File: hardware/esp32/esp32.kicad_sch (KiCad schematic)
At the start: 12 parts, among them J1 Conn_01x02, J2 Conn_01x02, J6 Conn_01x08, U2 ESP32-S3-MINI-1-N8

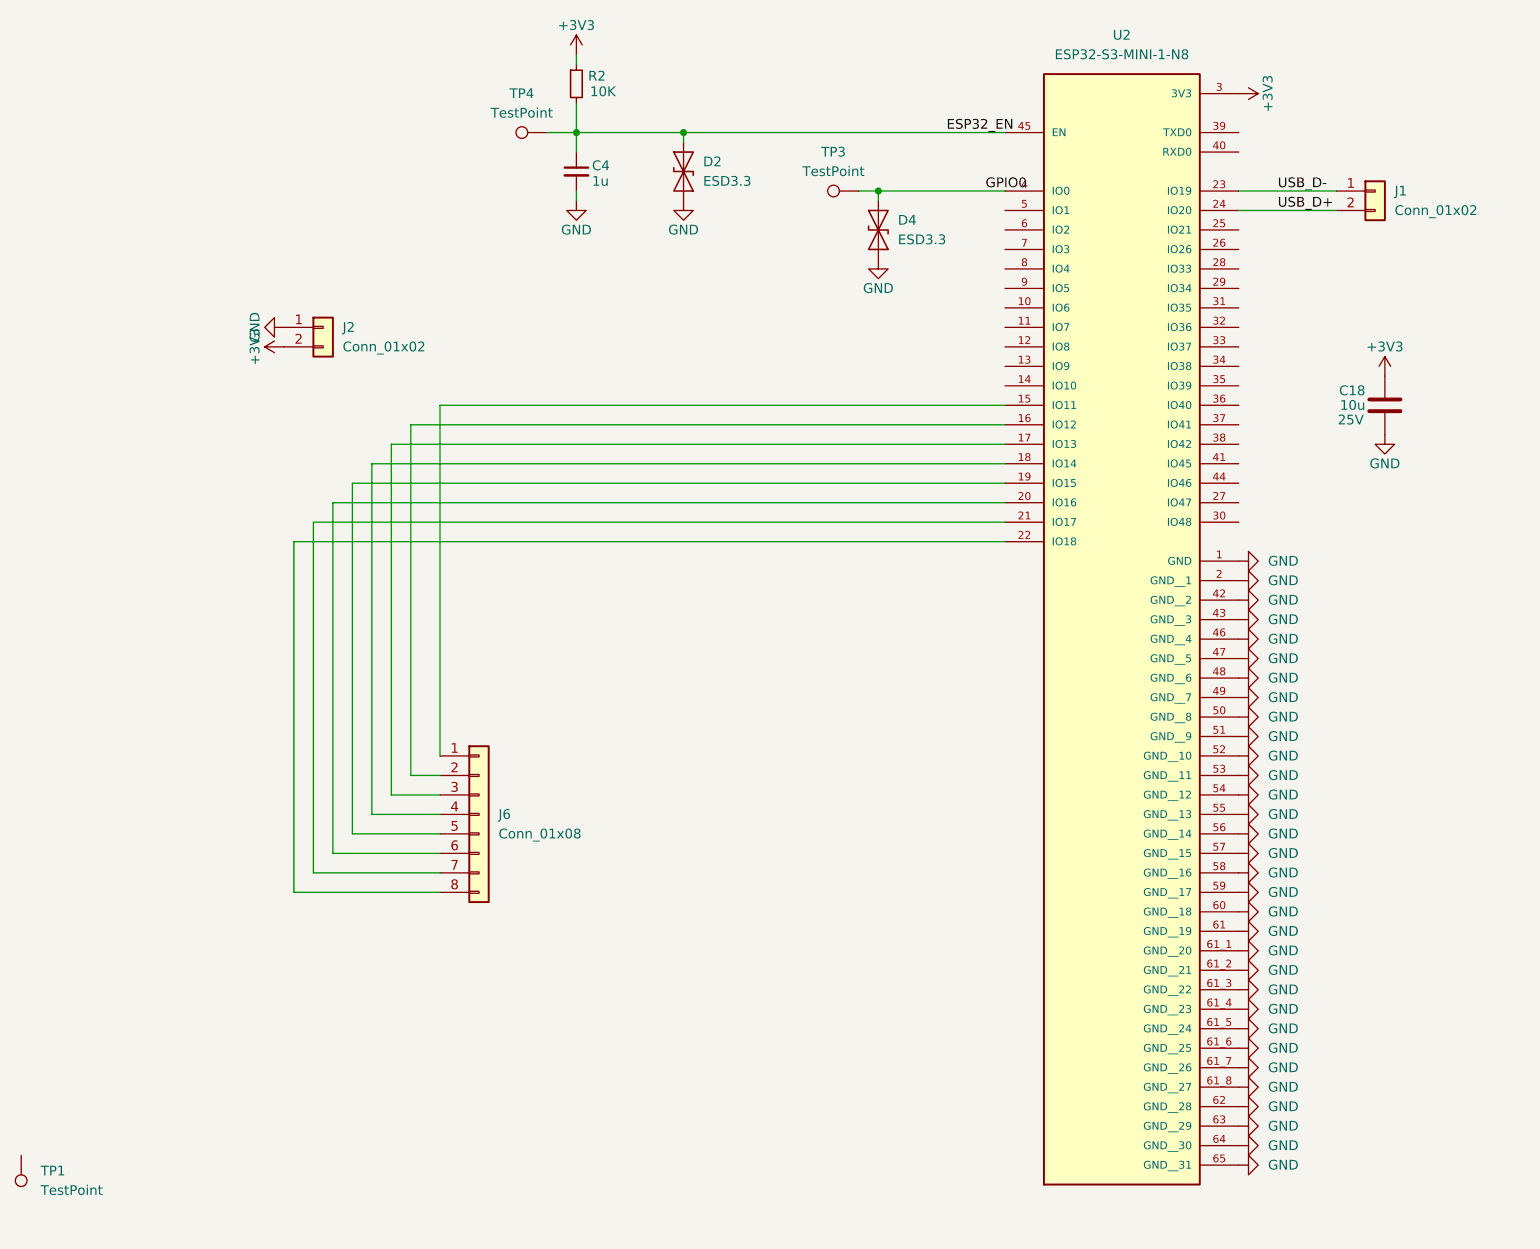
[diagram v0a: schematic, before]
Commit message: esp32 rebuild connectors
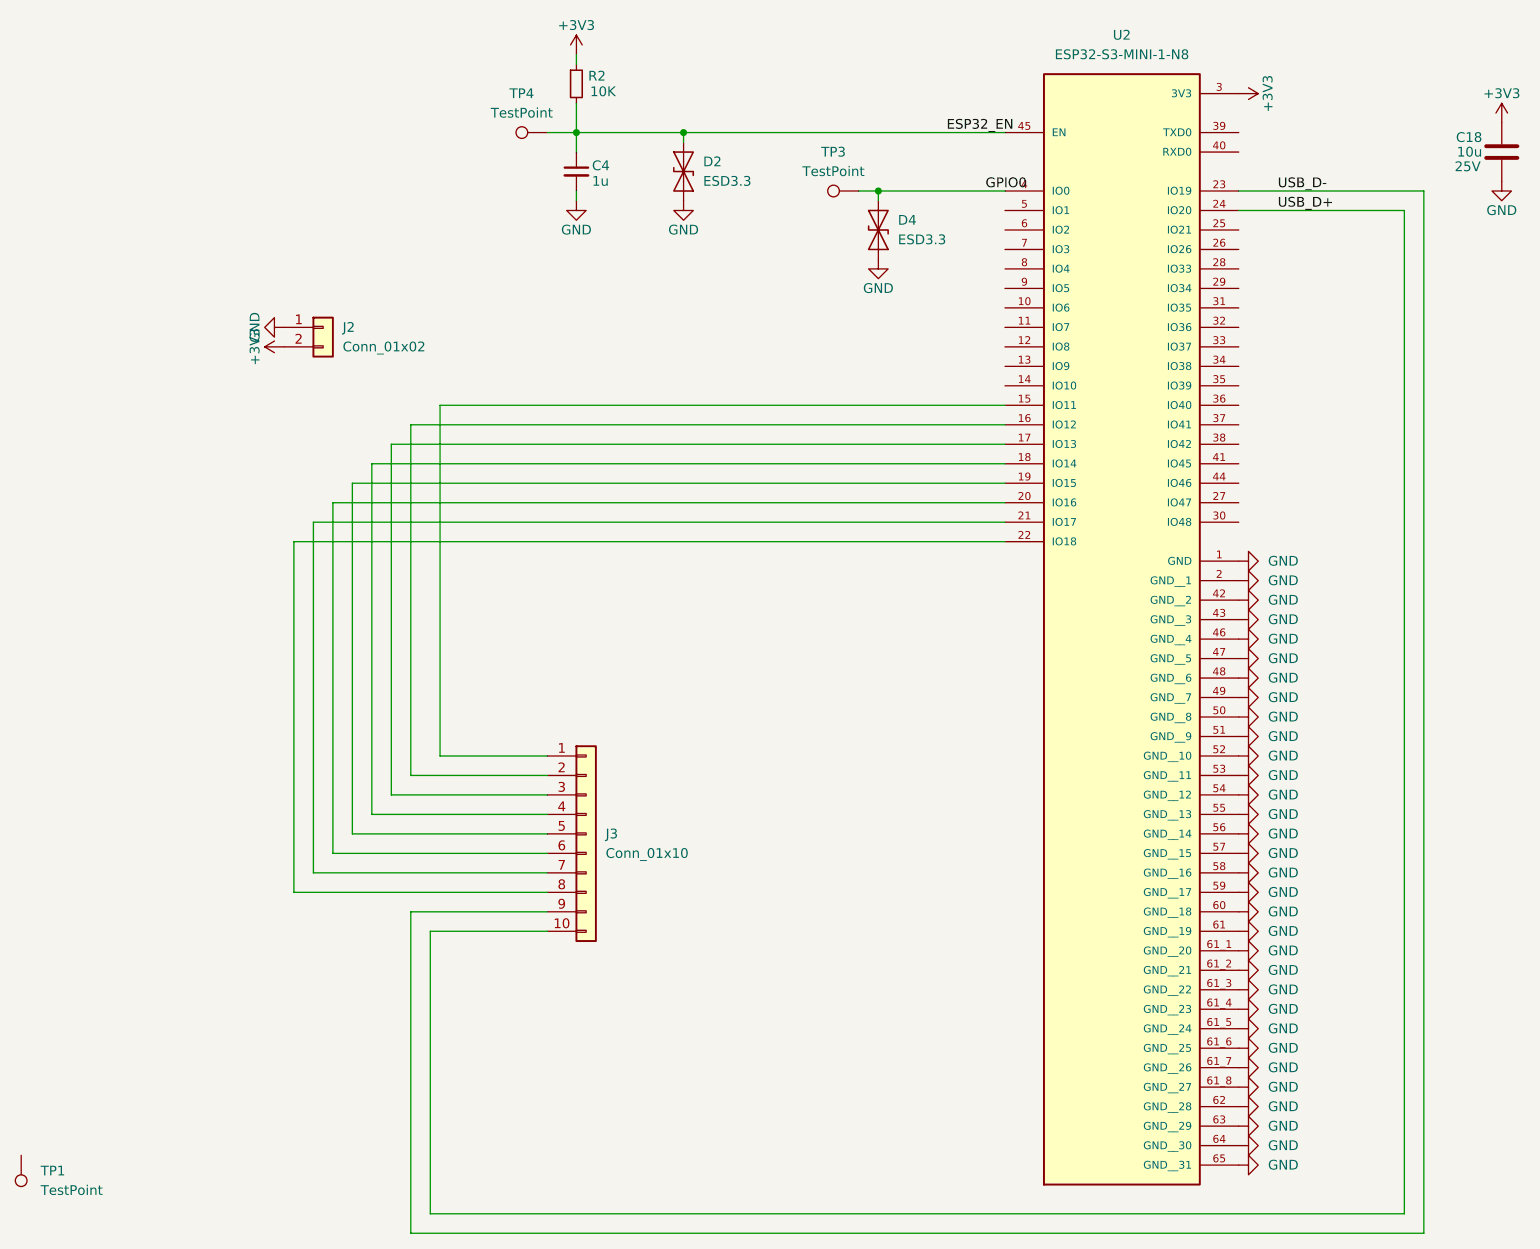
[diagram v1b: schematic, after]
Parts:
- removed J1: Conn_01x02, Connector_JST:JST_SHL_SM02B-SHLS-TF_1x02-1MP_P1.00mm_Horizontal, symbol Connector_Generic:Conn_01x02
- removed J6: Conn_01x08, Connector_JST:JST_SHL_SM08B-SHLS-TF_1x08-1MP_P1.00mm_Horizontal, symbol Connector_Generic:Conn_01x08
- added J3: Conn_01x10, Connector_JST:JST_SHL_SM10B-SHLS-TF_1x10-1MP_P1.00mm_Horizontal, symbol Connector_Generic:Conn_01x10
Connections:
- net USB_D+: now also J3.10 (Pin_10)
- net USB_D-: now also J3.9 (Pin_9)
- net at U2.15 (IO11): now also J3.1 (Pin_1)
- net at U2.16 (IO12): now also J3.2 (Pin_2)
- net at U2.17 (IO13): now also J3.3 (Pin_3)
- net at U2.18 (IO14): now also J3.4 (Pin_4)
- net at U2.19 (IO15): now also J3.5 (Pin_5)
- net at U2.20 (IO16): now also J3.6 (Pin_6)
- net at U2.21 (IO17): now also J3.7 (Pin_7)
- net at U2.22 (IO18): now also J3.8 (Pin_8)
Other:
- moved on the sheet: C18
